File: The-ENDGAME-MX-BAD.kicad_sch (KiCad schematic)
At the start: 78 parts, among them J1 Conn_01x04, SW1 SW_Push, SW10 SW_Push, SW11 SW_Push, SW12 SW_Push, SW13 SW_Push, SW14 SW_Push, SW15 SW_Push, SW16 SW_Push, SW17 SW_Push, SW18 SW_Push, SW19 SW_Push, SW2 SW_Push, SW20 SW_Push, SW21 SW_Push, SW22 SW_Push, SW23 SW_Push, SW24 SW_Push, SW25 SW_Push, SW26 SW_Push, SW27 SW_Push, SW28 SW_Push, SW29 SW_Push, SW3 SW_Push, SW30 SW_Push, SW31 SW_Push, SW32 SW_Push, SW33 SW_Push, SW34 SW_Push, SW35 SW_Push, SW36 SW_Push, SW4 SW_Push, SW5 SW_Push, SW6 SW_Push, SW7 SW_Push, SW8 SW_Push, SW9 SW_Push, U1 ProMicro-kbd-34key

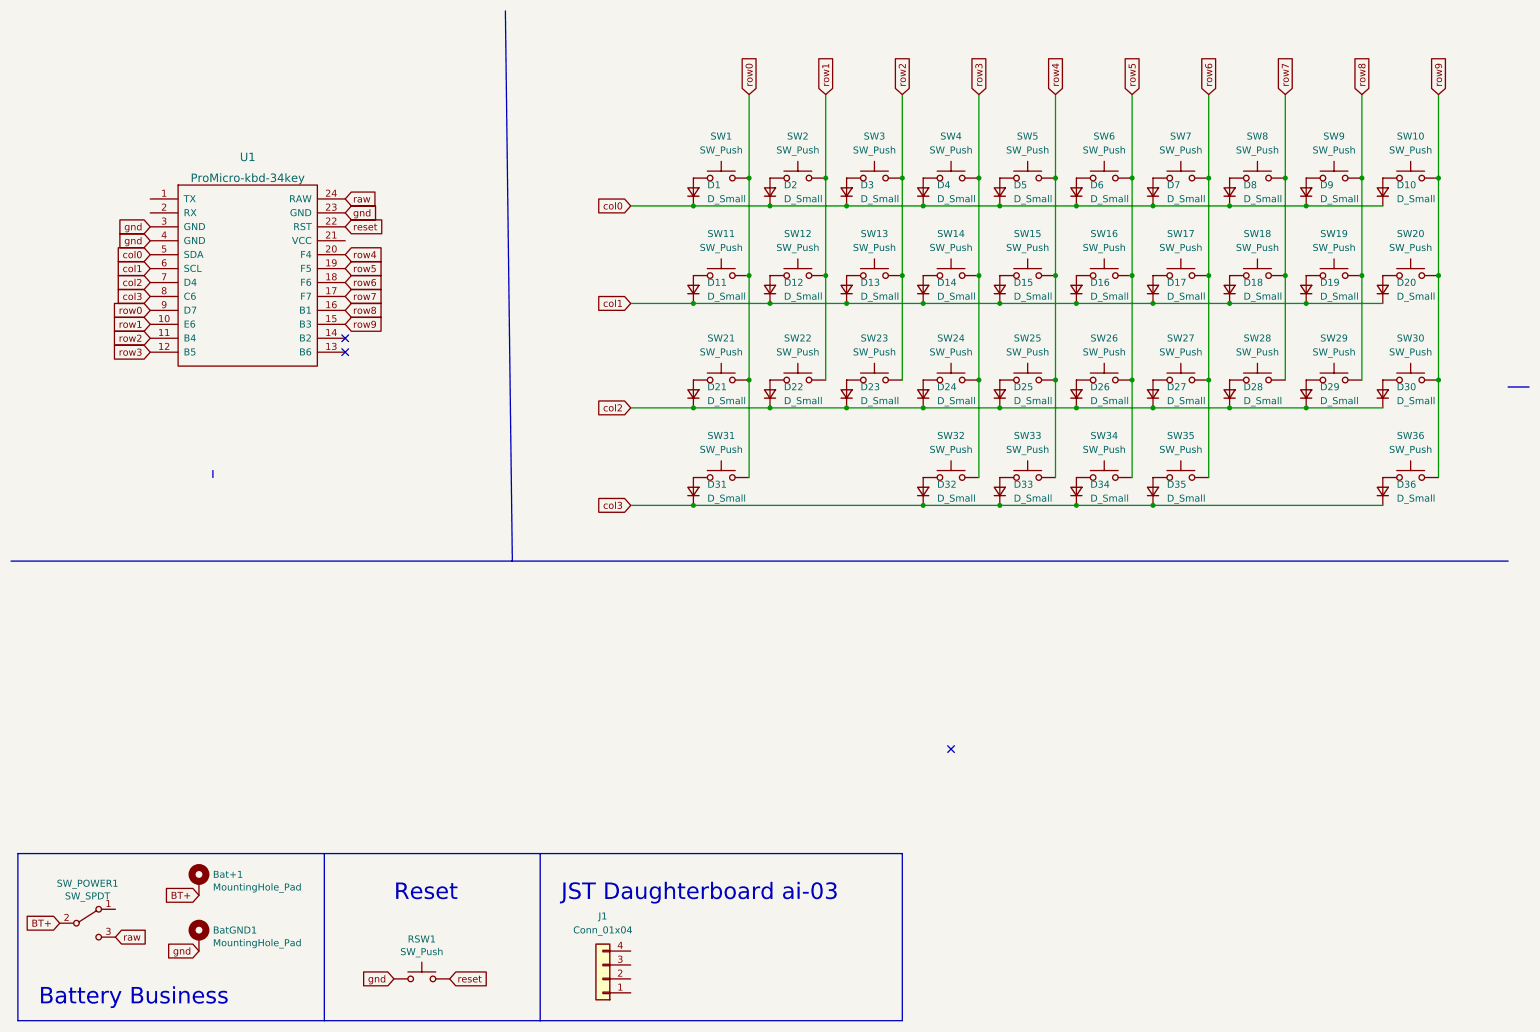
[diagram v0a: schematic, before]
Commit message: fast fertig
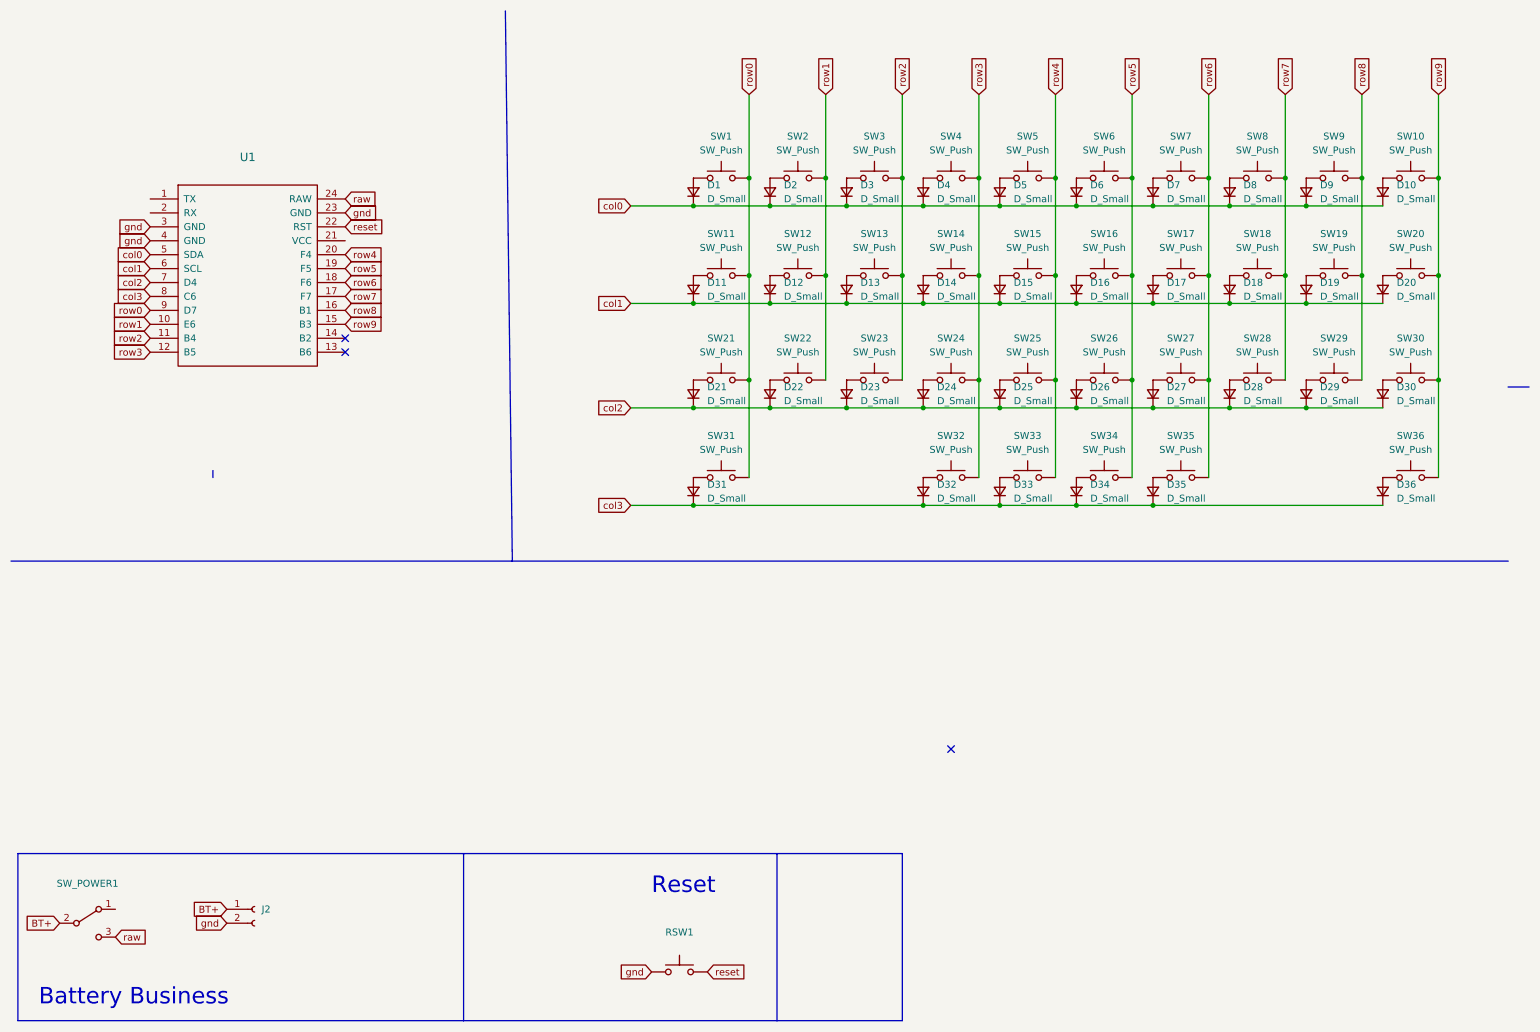
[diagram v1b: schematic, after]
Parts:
- removed Bat+1, BatGND1: MountingHole_Pad, kbd:1pin_conn, symbol Mechanical:MountingHole_Pad
- removed J1: Conn_01x04, Footprints:JST_SH_SM04B-SRSS-TB_1x04-1MP_P1.00mm_Horizontal, symbol ENDGAME_UWU_Gatekeeper_stuff:Conn_01x04
- added J2: (no value), symbol Connector:Conn_01x02_Female
- RSW1: value SW_Push -> (none); footprint kbd:ResetSW -> (none)
- SW_POWER1: value SW_SPDT -> (none); footprint Kailh:SPDT_C128955 -> (none)
- U1: value ProMicro-kbd-34key -> (none); footprint Keebio-Parts:ArduinoProMicro-BackSide -> (none)
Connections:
- net BT+: now also J2.1 (Pin_1)
- net gnd: now also J2.2 (Pin_2)
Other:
- note removed: "JST Daughterboard ai-03"
- moved on the sheet: RSW1

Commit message: pcb changes
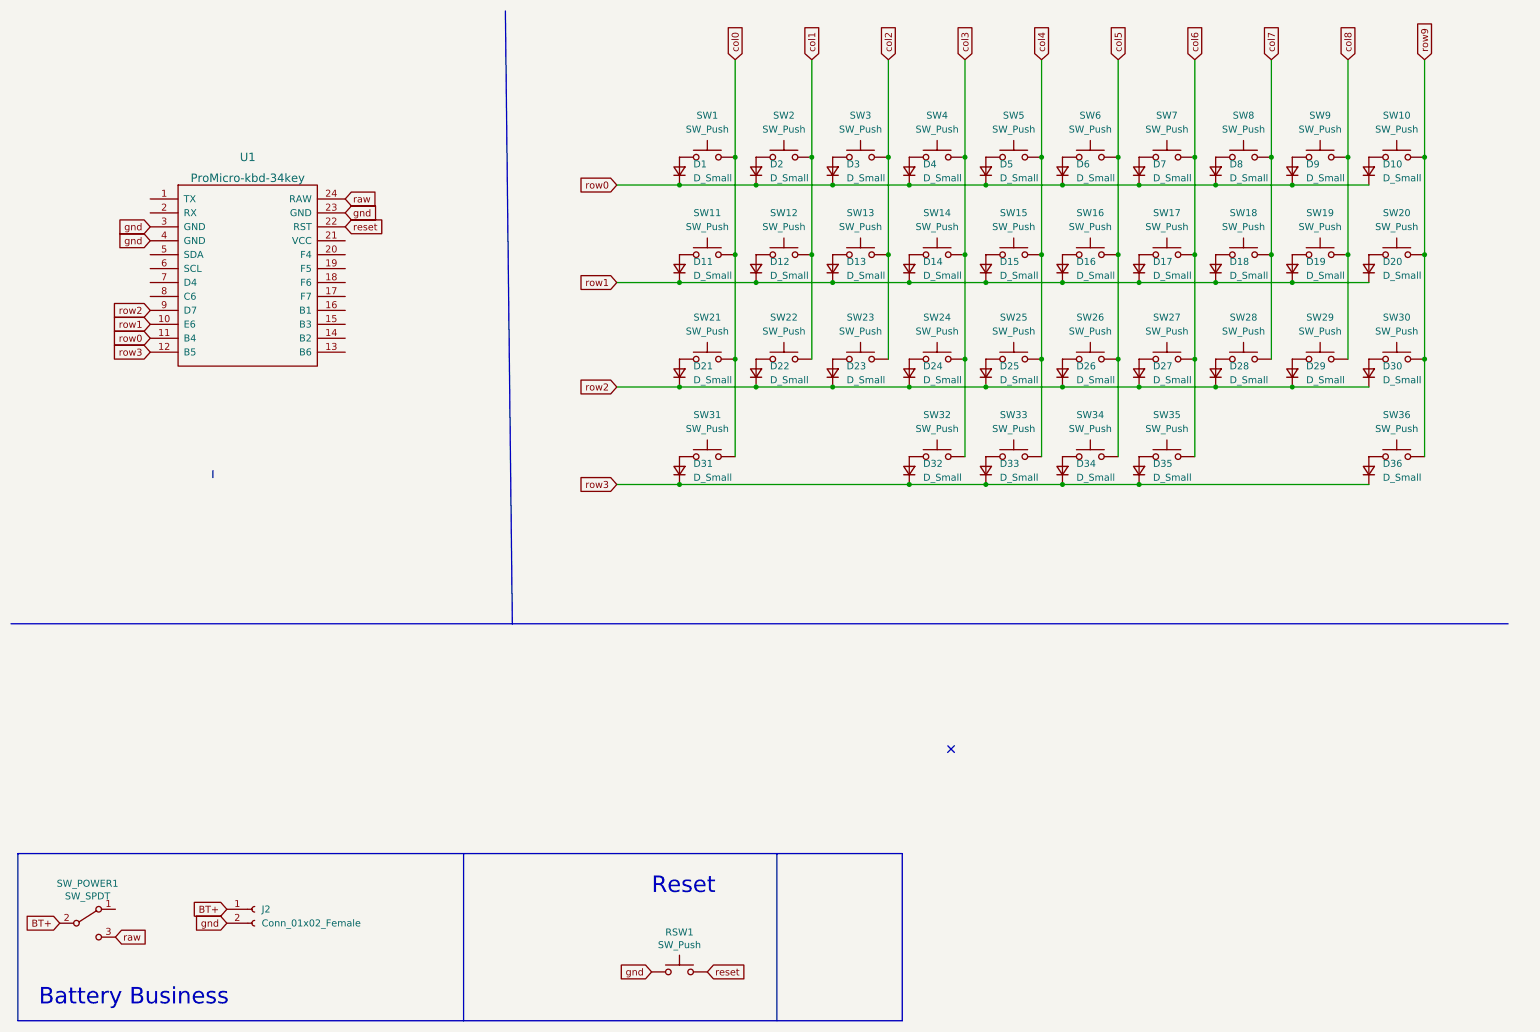
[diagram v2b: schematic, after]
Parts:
- J2: value (none) -> Conn_01x02_Female; footprint (none) -> Connector_JST:JST_SH_BM02B-SRSS-TB_1x02-1MP_P1.00mm_Vertical
- RSW1: value (none) -> SW_Push; footprint (none) -> Button_Switch_THT:SW_PUSH_6mm
- SW_POWER1: value (none) -> SW_SPDT; footprint (none) -> Button_Switch_SMD:SW_SPDT_PCM12
- U1: value (none) -> ProMicro-kbd-34key; footprint (none) -> Keebio-Parts:Elite-C-castellated-24pin-holes
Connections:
- net col0: now also SW1.2, SW11.2, SW21.2, SW31.2; no longer D1.1 (K), D10.1 (K), D2.1 (K), D3.1 (K), D4.1 (K), D5.1 (K), D6.1 (K), D7.1 (K), D8.1 (K), D9.1 (K), U1.5 (SDA)
- net col1: now also SW12.2, SW2.2, SW22.2; no longer D11.1 (K), D12.1 (K), D13.1 (K), D14.1 (K), D15.1 (K), D16.1 (K), D17.1 (K), D18.1 (K), D19.1 (K), D20.1 (K), U1.6 (SCL)
- net col2: now also SW13.2, SW23.2, SW3.2; no longer D21.1 (K), D22.1 (K), D23.1 (K), D24.1 (K), D25.1 (K), D26.1 (K), D27.1 (K), D28.1 (K), D29.1 (K), D30.1 (K), U1.7 (D4)
- net col3: now also SW14.2, SW24.2, SW32.2, SW4.2; no longer D31.1 (K), D32.1 (K), D33.1 (K), D34.1 (K), D35.1 (K), D36.1 (K), U1.8 (C6)
- net row0: now also D1.1 (K), D10.1 (K), D2.1 (K), D3.1 (K), D4.1 (K), D5.1 (K), D6.1 (K), D7.1 (K), D8.1 (K), D9.1 (K), U1.11 (B4); no longer SW1.2, SW11.2, SW21.2, SW31.2, U1.9 (D7)
- net row1: now also D11.1 (K), D12.1 (K), D13.1 (K), D14.1 (K), D15.1 (K), D16.1 (K), D17.1 (K), D18.1 (K), D19.1 (K), D20.1 (K); no longer SW12.2, SW2.2, SW22.2
- net row2: now also D21.1 (K), D22.1 (K), D23.1 (K), D24.1 (K), D25.1 (K), D26.1 (K), D27.1 (K), D28.1 (K), D29.1 (K), D30.1 (K), U1.9 (D7); no longer SW13.2, SW23.2, SW3.2, U1.11 (B4)
- net row3: now also D31.1 (K), D32.1 (K), D33.1 (K), D34.1 (K), D35.1 (K), D36.1 (K); no longer SW14.2, SW24.2, SW32.2, SW4.2
- net row9: no longer U1.15 (B3)
- net row4 renamed col4
- net col4: no longer U1.20 (F4)
- net row5 renamed col5
- net col5: no longer U1.19 (F5)
- net row6 renamed col6
- net col6: no longer U1.18 (F6)
- net row7 renamed col7
- net col7: no longer U1.17 (F7)
- net row8 renamed col8
- net col8: no longer U1.16 (B1)
- no-connect marks 3 -> 1
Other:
- moved on the sheet: D1, D10, D11, D12, D13, D14, D15, D16, D17, D18, D19, D2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

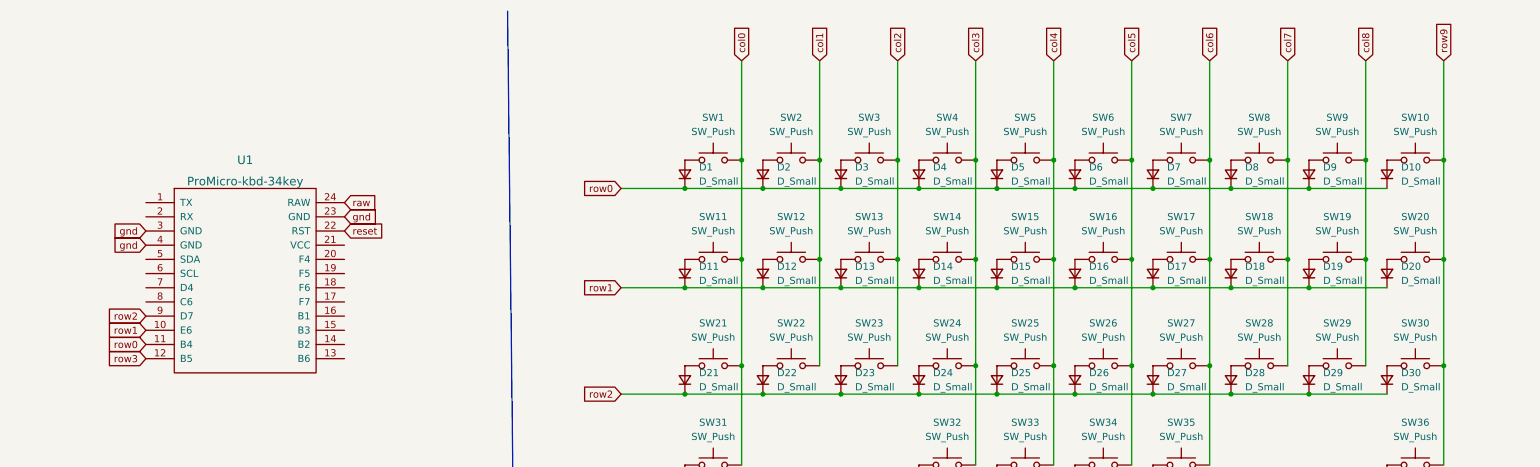
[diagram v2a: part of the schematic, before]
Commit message: soweit so gut ENDGAME outline und layout final
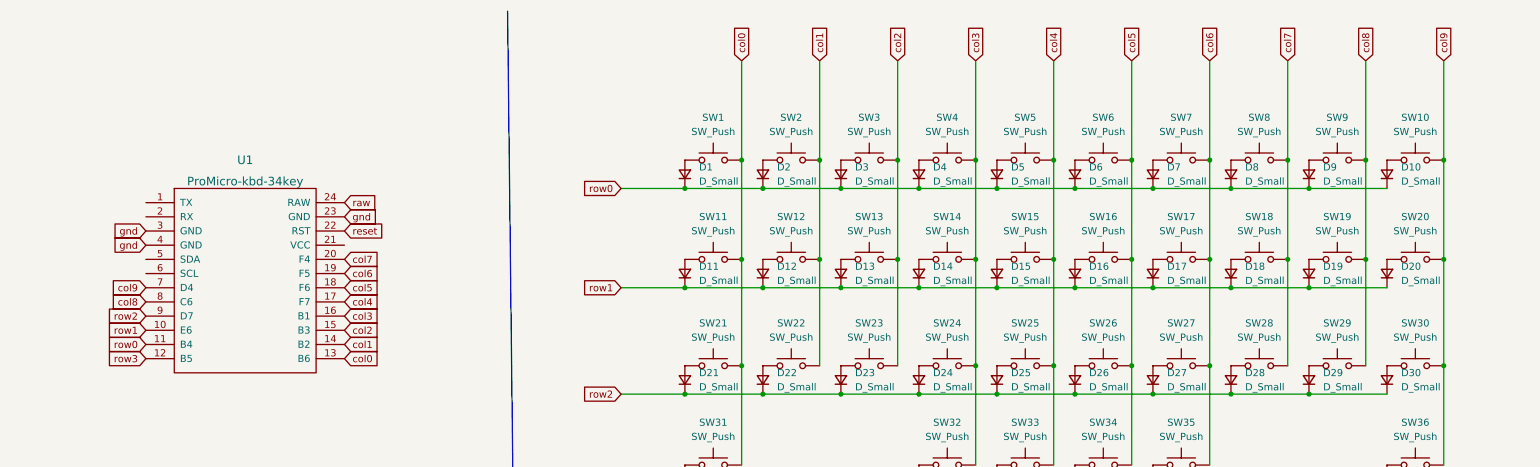
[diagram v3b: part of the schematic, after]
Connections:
- net row9 is gone; now on net col9: SW10.2, SW20.2, SW30.2, SW36.2
- net col0: now also U1.13 (B6)
- net col1: now also U1.14 (B2)
- net col2: now also U1.15 (B3)
- net col3: now also U1.16 (B1)
- net col4: now also U1.17 (F7)
- net col5: now also U1.18 (F6)
- net col6: now also U1.19 (F5)
- net col7: now also U1.20 (F4)
- net col8: now also U1.8 (C6)
- net col9: now reaches U1.7 (D4)
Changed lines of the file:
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@@
+    )
+  )
+  (global_label "col5" (shape input) (at 73.66 62.23 0) (fields_autoplaced)
+    (effects (font (size 1.27 1.27)) (justify left))
+    (property "Intersheet References" "${INTERSHEET_REFS}" (id 0) (at 80.1855 62.1506 0)
+      (effects (font (size 1.27 1.27)) (justify left) hide)
     )
   )
@@
     )
   )
+  (global_label "col7" (shape input) (at 73.66 57.15 0) (fields_autoplaced)
+    (effects (font (size 1.27 1.27)) (justify left))
+    (property "Intersheet References" "${INTERSHEET_REFS}" (id 0) (at 80.1855 57.0706 0)
+      (effects (font (size 1.27 1.27)) (justify left) hide)
+    )
+  )
   (global_label "row2" (shape input) (at 38.1 67.31 180) (fields_autoplaced)
     (effects (font (size 1.27 1.27)) (justify right))
@@
     )
   )
+  (global_label "col6" (shape input) (at 73.66 59.69 0) (fields_autoplaced)
+    (effects (font (size 1.27 1.27)) (justify left))
+    (property "Intersheet References" "${INTERSHEET_REFS}" (id 0) (at 80.1855 59.6106 0)
+      (effects (font (size 1.27 1.27)) (justify left) hide)
+    )
+  )
   (global_label "reset" (shape input) (at 73.66 52.07 0) (fields_autoplaced)
     (effects (font (size 1.27 1.27)) (justify left))
@@
     )
   )
+  (global_label "col1" (shape input) (at 73.66 72.39 0) (fields_autoplaced)
+    (effects (font (size 1.27 1.27)) (justify left))
+    (property "Intersheet References" "${INTERSHEET_REFS}" (id 0) (at 80.1855 72.3106 0)
+      (effects (font (size 1.27 1.27)) (justify left) hide)
+    )
+  )
   (global_label "BT+" (shape input) (at 21.59 179.07 180) (fields_autoplaced)
     (effects (font (size 1.27 1.27)) (justify right))
@@
     )
   )
+  (global_label "col4" (shape input) (at 73.66 64.77 0) (fields_autoplaced)
+    (effects (font (size 1.27 1.27)) (justify left))
+    (property "Intersheet References" "${INTERSHEET_REFS}" (id 0) (at 80.1855 64.6906 0)
+      (effects (font (size 1.27 1.27)) (justify left) hide)
+    )
+  )
   (global_label "row2" (shape input) (at 123.19 81.28 180) (fields_autoplaced)
     (effects (font (size 1.27 1.27)) (justify right))
@@
     )
   )
-  (global_label "row9" (shape input) (at 270.51 21.59 90) (fields_autoplaced)
-    (effects (font (size 1.27 1.27)) (justify left))
-    (property "Intersheet References" "${INTERSHEET_REFS}" (id 0) (at 270.4306 14.7017 90)
+  (global_label "col9" (shape input) (at 270.51 21.59 90) (fields_autoplaced)
+    (effects (font (size 1.27 1.27)) (justify left))
+    (property "Intersheet References" "${INTERSHEET_REFS}" (id 0) (at 270.4306 15.0645 90)
       (effects (font (size 1.27 1.27)) (justify left) hide)
     )
@@
     )
   )
+  (global_label "col2" (shape input) (at 73.66 69.85 0) (fields_autoplaced)
+    (effects (font (size 1.27 1.27)) (justify left))
+    (property "Intersheet References" "${INTERSHEET_REFS}" (id 0) (at 80.1855 69.7706 0)
+      (effects (font (size 1.27 1.27)) (justify left) hide)
+    )
+  )
   (global_label "gnd" (shape input) (at 52.07 179.07 180) (fields_autoplaced)
     (effects (font (size 1.27 1.27)) (justify right))
@@
     )
   )
+  (global_label "col3" (shape input) (at 73.66 67.31 0) (fields_autoplaced)
+    (effects (font (size 1.27 1.27)) (justify left))
+    (property "Intersheet References" "${INTERSHEET_REFS}" (id 0) (at 80.1855 67.2306 0)
+      (effects (font (size 1.27 1.27)) (justify left) hide)
+    )
+  )
   (global_label "raw" (shape input) (at 73.66 46.99 0) (fields_autoplaced)
     (effects (font (size 1.27 1.27)) (justify left))
@@
     )
   )
+  (global_label "col0" (shape input) (at 73.66 74.93 0) (fields_autoplaced)
+    (effects (font (size 1.27 1.27)) (justify left))
+    (property "Intersheet References" "${INTERSHEET_REFS}" (id 0) (at 80.1855 74.8506 0)
+      (effects (font (size 1.27 1.27)) (justify left) hide)
+    )
+  )
+  (global_label "col8" (shape input) (at 38.1 64.77 180) (fields_autoplaced)
+    (effects (font (size 1.27 1.27)) (justify right))
+    (property "Intersheet References" "${INTERSHEET_REFS}" (id 0) (at 31.5745 64.8494 0)
+      (effects (font (size 1.27 1.27)) (justify right) hide)
+    )
+  )
   (global_label "col6" (shape input) (at 228.6 21.59 90) (fields_autoplaced)
     (effects (font (size 1.27 1.27)) (justify left))
@@
     )
   )
+  (global_label "col9" (shape input) (at 38.1 62.23 180) (fields_autoplaced)
+    (effects (font (size 1.27 1.27)) (justify right))
+    (property "Intersheet References" "${INTERSHEET_REFS}" (id 0) (at 31.5745 62.3094 0)
+      (effects (font (size 1.27 1.27)) (justify right) hide)
+    )
+  )
